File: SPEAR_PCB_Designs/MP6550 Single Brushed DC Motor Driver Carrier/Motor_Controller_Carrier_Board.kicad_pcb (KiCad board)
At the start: 2 copper layers, 88.6 x 47.3 mm, 19 parts, among them J1 Conn_01x02_Pin, J2 Conn_01x02_Pin, J3 Conn_01x02_Pin, J4 Conn_01x04_Pin, U1 AP63203WU

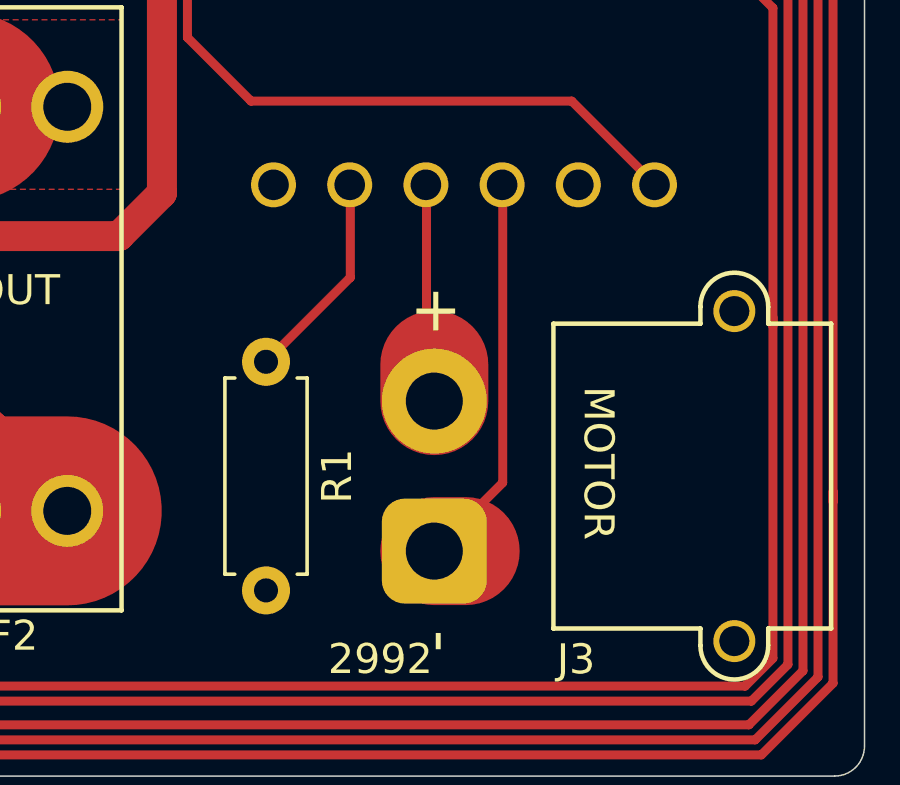
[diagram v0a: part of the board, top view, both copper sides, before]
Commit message: Update Motor_Controller_Carrier_Board.kicad_pcb
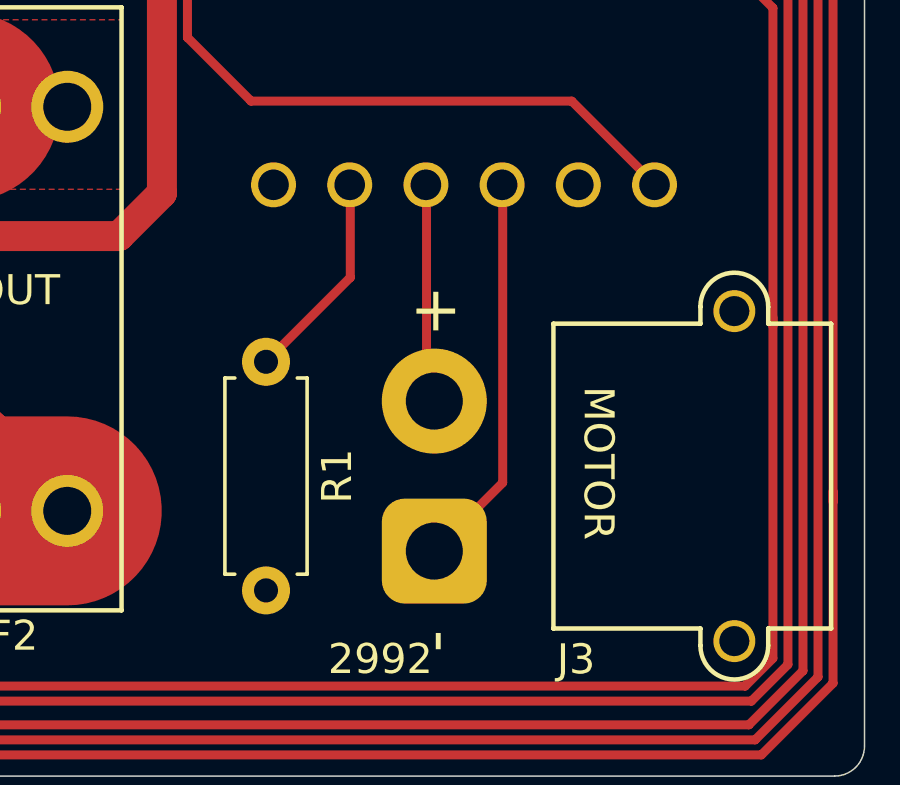
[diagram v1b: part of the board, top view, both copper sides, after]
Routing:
- net Net-(J3-Pin_2): track 5.37 -> 7.33 mm
- net Net-(J3-Pin_1): track 15.5 -> 14.5 mm
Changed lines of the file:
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@@
+	)
+	(segment
+		(start 158.35 103.24)
+		(end 158.61 103.5)
+		(width 0.3)
+		(layer "F.Cu")
+		(net 1)
 	)
 	(segment
 		(start 158.35 96.28)
-		(end 158.35 100.435558)
-		(width 0.3)
-		(layer "F.Cu")
-		(net 1)
-	)
-	(segment
-		(start 158.61 103.5)
-		(end 158.61 102.285558)
-		(width 3.6)
+		(end 158.35 103.24)
+		(width 0.3)
 		(layer "F.Cu")
 		(net 1)
@@
 		(layer "F.Cu")
 		(net 11)
-	)
-	(segment
-		(start 158.61 108.5)
-		(end 159.655558 108.5)
-		(width 3.6)
-		(layer "F.Cu")
-		(net 11)
